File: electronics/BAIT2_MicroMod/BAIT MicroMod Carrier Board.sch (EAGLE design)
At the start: 109 parts, among them J1 microSD, J4 JST_6_PIN_VERTICAL, J5 QWIIC_RIGHT_ANGLE, U3 3.3V, U4 3.3V, U5 BQ27441-G1, X1 2.1mm DC, X2 BQ24074

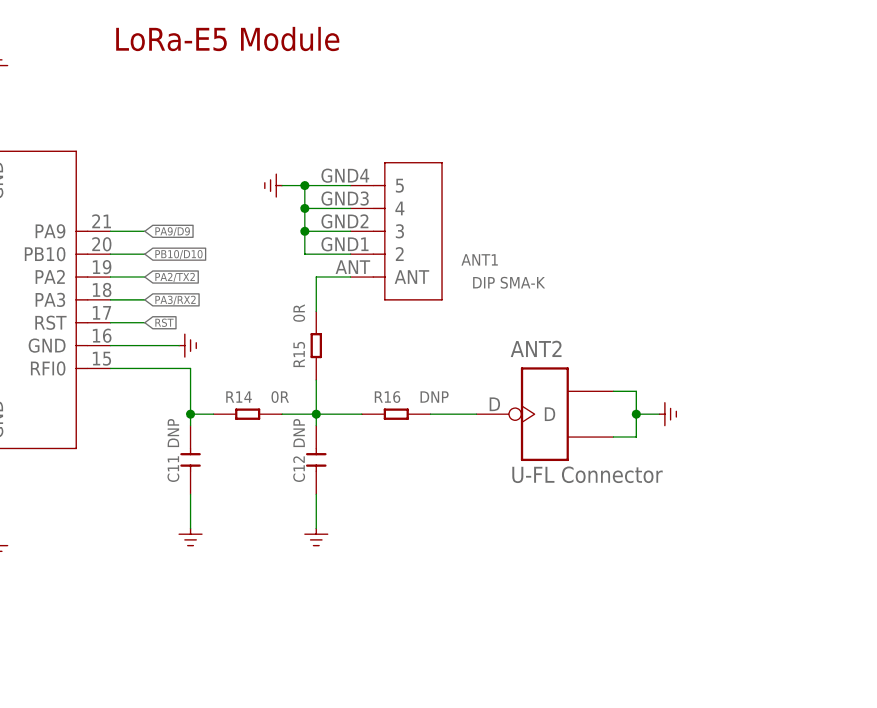
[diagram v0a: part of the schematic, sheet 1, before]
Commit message: Board layout updates
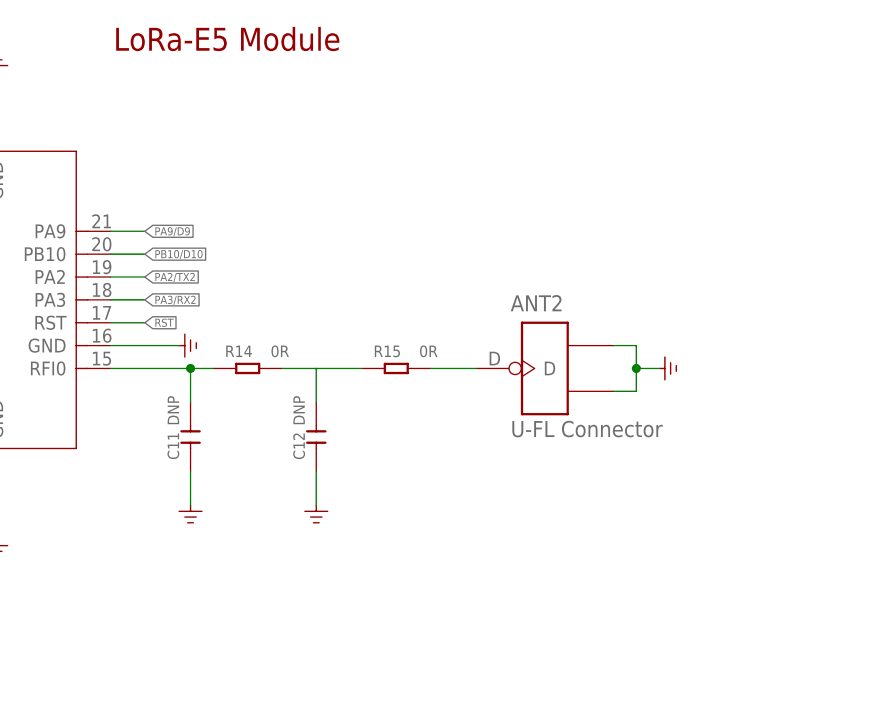
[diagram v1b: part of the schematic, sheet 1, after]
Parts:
- removed ANT1: DIP SMA-K, Connector-new:ANTENNA-SMA-MCX-JE-320160125
- removed R16: DNP, Discrete-new:RES-0402
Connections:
- removed net N$10: ANT2.D, R16.2
- removed net N$13: ANT1.ANT, R15.2
- new net N$7: ANT2.D, R15.2
- net GND: no longer ANT1.2, ANT1.3, ANT1.4, ANT1.5
- net N$28: no longer R16.1
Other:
- moved on the sheet: ANT2, C11, C12, R14, R15
